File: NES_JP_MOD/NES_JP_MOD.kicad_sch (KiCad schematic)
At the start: 9 parts, among them J1 Conn_01x06, U1 XC2C64A, U2 AMS1117-1.8, U3 AMS1117-3.3, X1 ASV-xxxMHz

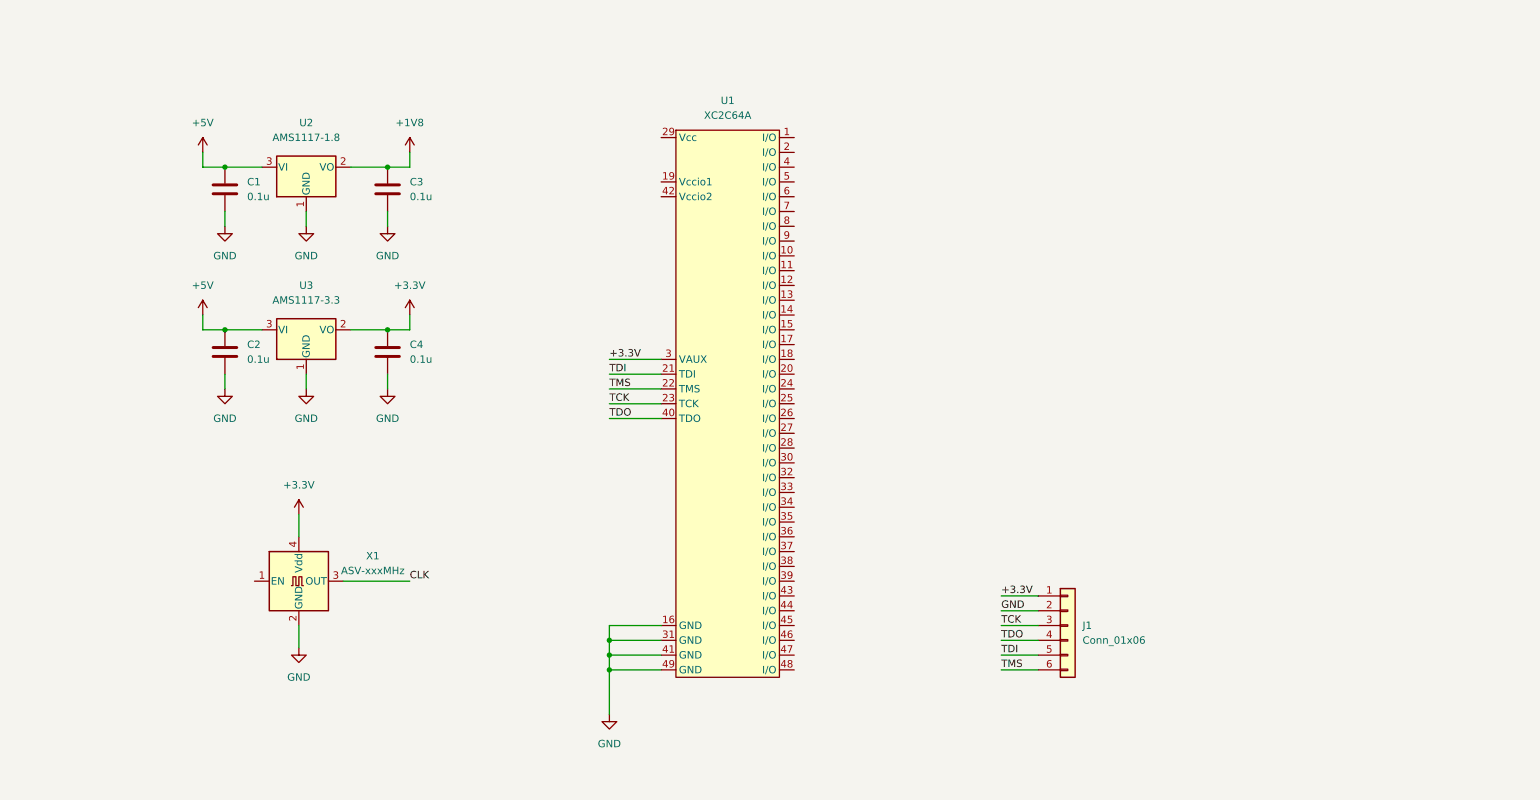
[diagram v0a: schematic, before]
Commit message: Created PCB
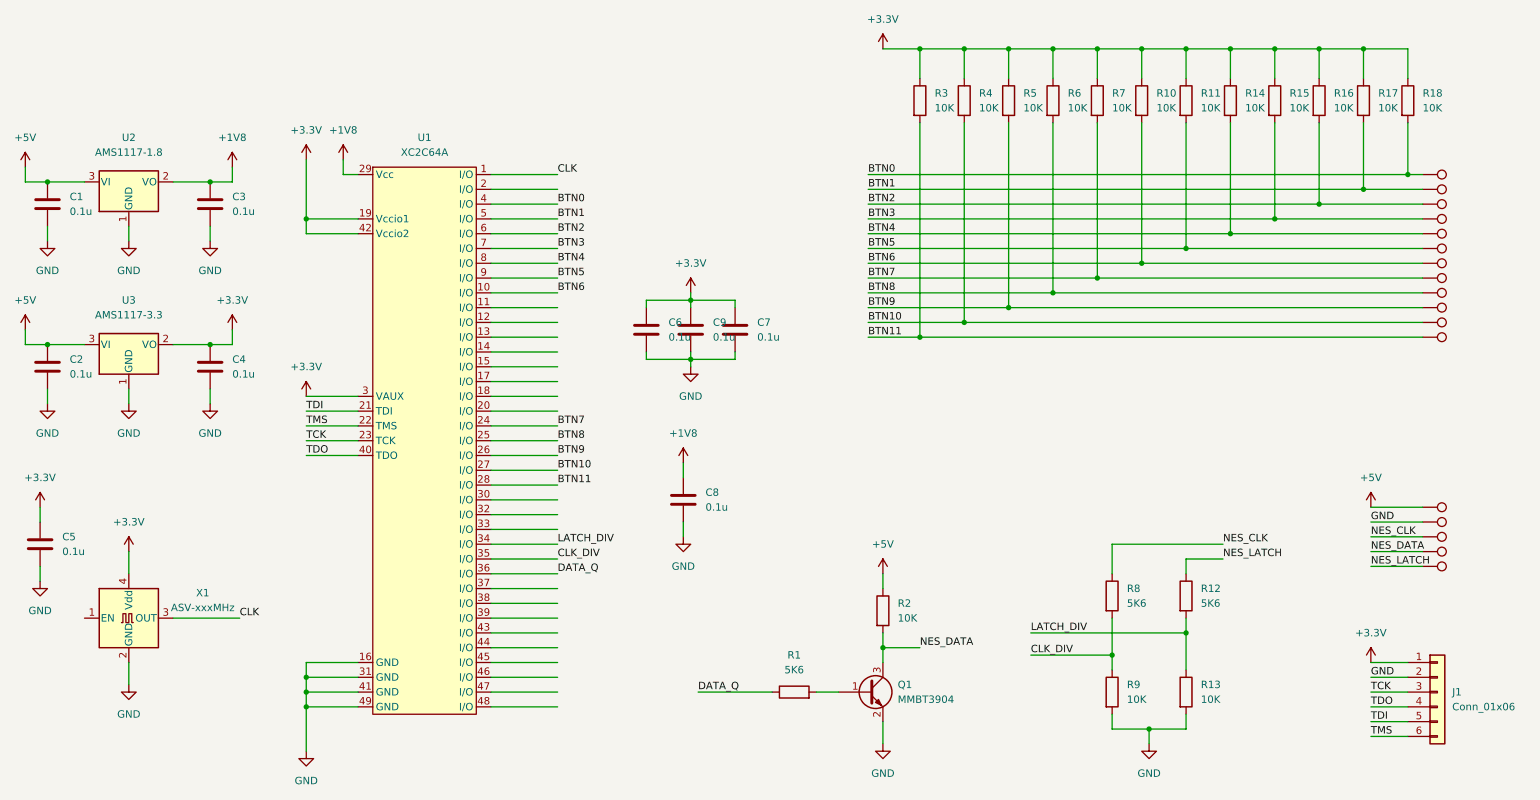
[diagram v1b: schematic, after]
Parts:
- added C5, C6, C7, C8, C9: 0.1u, Capacitor_SMD:C_0805_2012Metric, symbol Device:C
- added Q1: MMBT3904, Package_TO_SOT_SMD:SOT-23, symbol Transistor_BJT:MMBT3904
- added R1, R12, R8: 5K6, Resistor_SMD:R_0805_2012Metric, symbol Device:R
- added R10, R11, R13, R14, R15, R16, R17, R18, R2, R3, R4, R5, R6, R7, R9: 10K, Resistor_SMD:R_0805_2012Metric, symbol Device:R
- added TP1, TP10, TP11, TP12, TP13, TP14, TP15, TP16, TP17, TP2, TP3, TP4, TP5, TP6, TP7, TP8, TP9: TestPoint, TestPoint:TestPoint_Pad_2.0x2.0mm, symbol Connector:TestPoint
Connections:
- net +3.3V is gone; now on net +3V3: C4.1, J1.1 (Pin_1), U1.3 (VAUX), U3.2 (VO), X1.4 (Vdd)
- net +1V8: now also U1.29 (Vcc), C8.1
- net +5V: now also R2.1, TP16.1
- net CLK: now also U1.1 (I/O)
- net GND: now also C5.2, C6.2, C7.2, C8.2, C9.2, Q1.2 (E), R13.2, R9.2, TP17.1
- net BTN6: now reaches U1.10 (I/O)
- net BTN6: now also R10.2, TP8.1
- net +3V3: now reaches U1.19 (Vccio1)
- net +3V3: now also U1.42 (Vccio2), C5.1, C6.1, C7.1, C9.1, R10.1, R11.1, R14.1, R15.1, R16.1, R17.1, R18.1, R3.1, R4.1, R5.1, R6.1, R7.1
- net BTN7: now reaches U1.24 (I/O)
- net BTN7: now also R7.2, TP9.1
- net BTN8: now reaches U1.25 (I/O)
- net BTN8: now also R6.2, TP10.1
- net BTN9: now reaches U1.26 (I/O)
- net BTN9: now also R5.2, TP11.1
- net BTN10: now reaches U1.27 (I/O)
- net BTN10: now also R4.2, TP12.1
- net BTN11: now reaches U1.28 (I/O)
- net BTN11: now also R3.2, TP13.1
- net LATCH_DIV: now reaches U1.34 (I/O)
- net LATCH_DIV: now also R12.2, R13.1
- net CLK_DIV: now reaches U1.35 (I/O)
- net CLK_DIV: now also R8.2, R9.1
- net DATA_Q: now reaches U1.36 (I/O)
- net DATA_Q: now also R1.1
- net BTN0: now reaches U1.4 (I/O)
- net BTN0: now also R18.2, TP2.1
- net BTN1: now reaches U1.5 (I/O)
- net BTN1: now also R17.2, TP3.1
- net BTN2: now reaches U1.6 (I/O)
- net BTN2: now also R16.2, TP4.1
- net BTN3: now reaches U1.7 (I/O)
- net BTN3: now also R15.2, TP5.1
- net BTN4: now reaches U1.8 (I/O)
- net BTN4: now also R14.2, TP6.1
- net BTN5: now reaches U1.9 (I/O)
- net BTN5: now also R11.2, TP7.1
- new net: Q1.1 (B), R1.2
- new net NES_CLK: R8.1, TP14.1
- new net NES_DATA: Q1.3 (C), R2.2, TP1.1
- new net NES_LATCH: R12.1, TP15.1
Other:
- moved on the sheet: C1, C2, C3, C4, J1, U1, U2, U3, X1
